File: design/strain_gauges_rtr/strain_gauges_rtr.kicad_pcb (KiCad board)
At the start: 2 copper layers, 88.9 x 44.5 mm, 41 parts, among them J1 Conn_01x03, J2 Conn_01x03, J3 Conn_01x08, J4 Conn_01x04, J5 Conn_01x04, J6 Conn_01x04, J7 Conn_01x04, P1 CONN_01X02, Q1 2N3096, U1 TL780-15, U2 LT1460-10, U3 INA826, U4 INA826, U5 INA826, U6 INA826

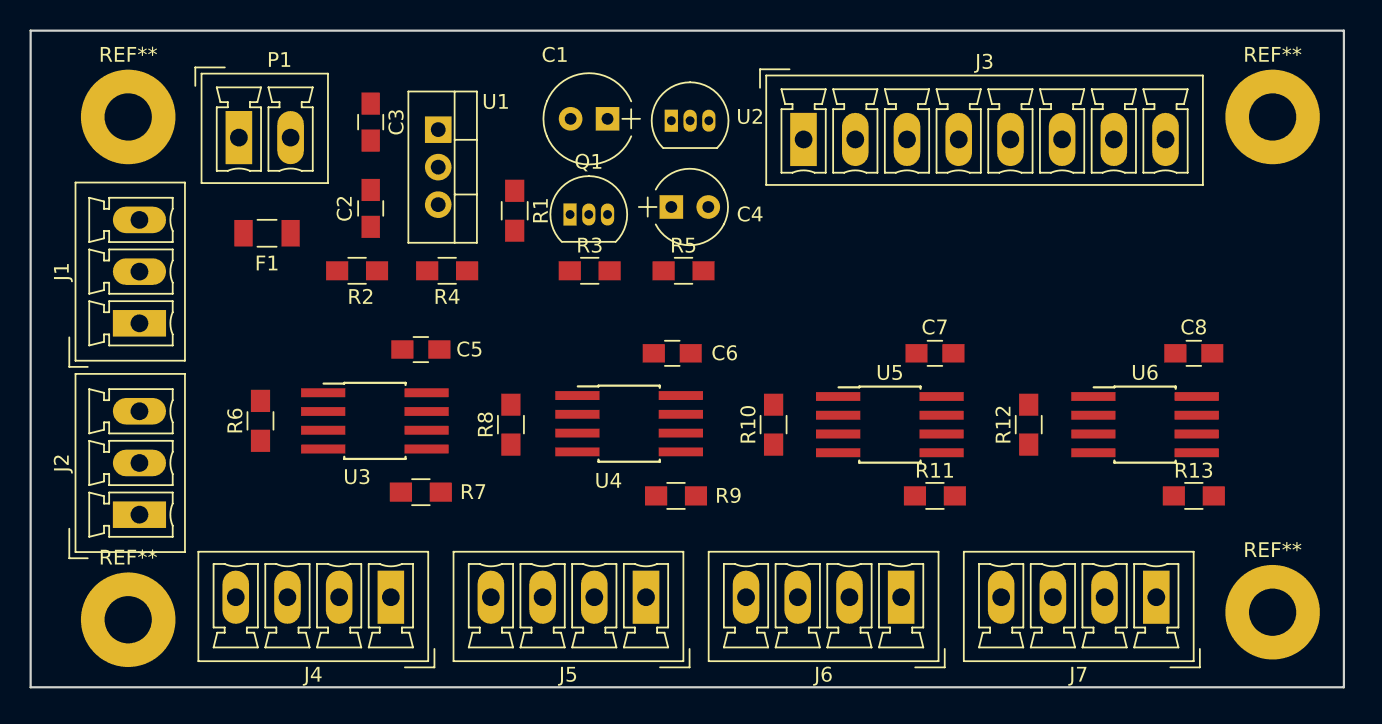
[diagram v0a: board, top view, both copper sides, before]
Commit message: Finish routing on INA826 board.
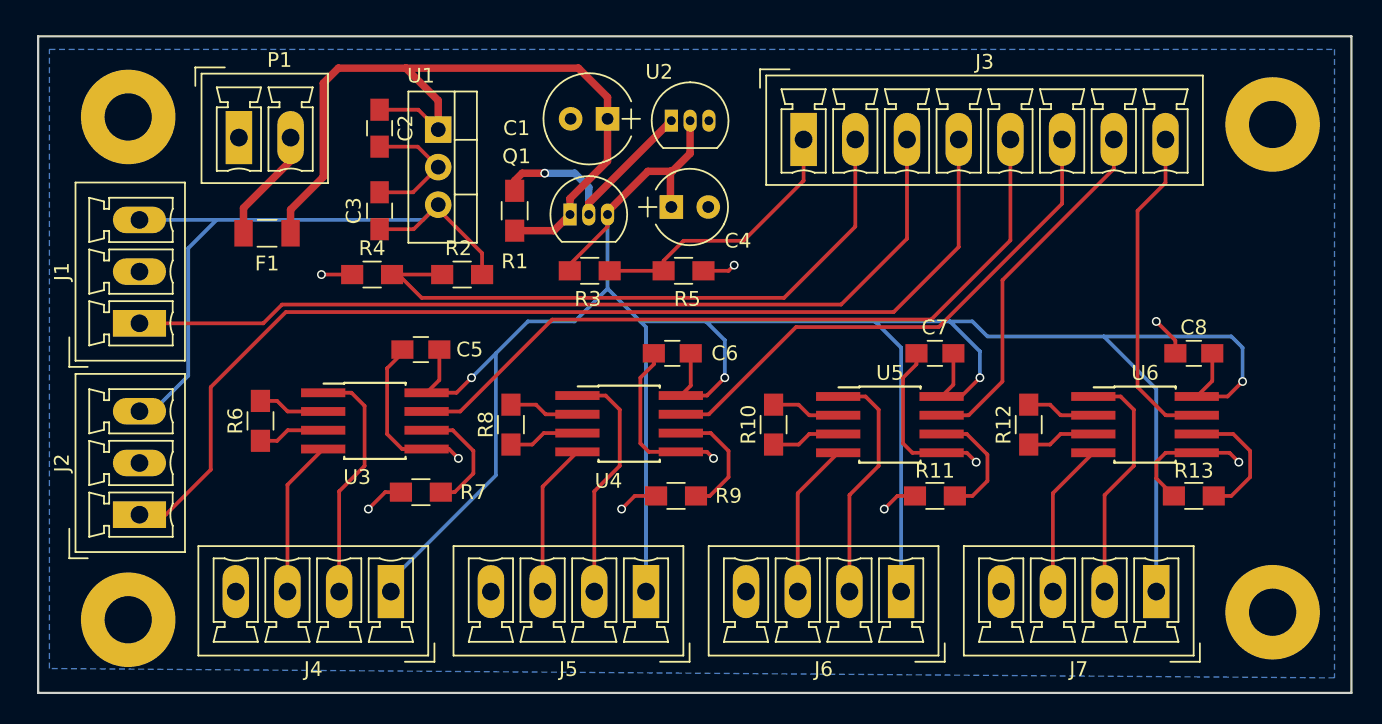
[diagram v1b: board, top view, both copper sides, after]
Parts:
- moved R2 7.12 mm to (118.4, 105.9), turned to 180 degrees
- moved C3 6.03 mm to (112.8, 101.6), turned to 90 degrees
- moved C2 5.46 mm to (112.8, 96.0), turned to 270 degrees
- moved R4 5.09 mm to (112.3, 105.9), turned to 180 degrees
- moved REF** 0.51 mm to (173.2, 95.8)
- moved J4 0.38 mm to (113.5, 127.4)
- moved J5 0.38 mm to (130.8, 127.4)
- moved J6 0.38 mm to (148.1, 127.4)
- moved J7 0.38 mm to (165.4, 127.4)
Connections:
- J3 pad 3: /PRESSURE_2 -> /PRESSURE_1
- J3 pad 4: /PRESSURE_1 -> /PRESSURE_2
- J3 pad 5: /STRAIN_OUT_4 -> /STRAIN_OUT_1
- J3 pad 6: /STRAIN_OUT_3 -> /STRAIN_OUT_2
- J3 pad 7: /STRAIN_OUT_2 -> /STRAIN_OUT_3
- J3 pad 8: /STRAIN_OUT_1 -> /STRAIN_OUT_4
- U4 pad 7: /STRAIN_OUT_3 -> /STRAIN_OUT_2
- U5 pad 7: /STRAIN_OUT_2 -> /STRAIN_OUT_3
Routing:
- net +10V: track 0.00 -> 191.5 mm, vias 0 -> 4
- net /PRESSURE_2: track 0.00 -> 73.5 mm
- net GND: track 0.00 -> 68.4 mm, vias 0 -> 10
- net /PRESSURE_1: track 0.00 -> 61.0 mm
- net +16V: track 0.00 -> 54.3 mm
- net /STRAIN_OUT_1: track 0.00 -> 51.1 mm
- net +15V: track 0.00 -> 46.9 mm
- net Net-(J3-Pad2): track 0.00 -> 43.3 mm
- net /STRAIN_OUT_2: track 0.00 -> 36.1 mm
- net /STRAIN_OUT_3: track 0.00 -> 24.6 mm
- net /STRAIN_OUT_4: track 0.00 -> 22.3 mm
- net Net-(J3-Pad1): track 0.00 -> 18.8 mm
- net Net-(Q1-Pad2): track 0.00 -> 16.8 mm, vias 0 -> 1
- net Net-(J4-Pad2): track 0.00 -> 16.5 mm
- net Net-(J5-Pad2): track 0.00 -> 16.3 mm
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- added copper zone on B.Cu, net GND
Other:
- rule pad_to_mask_clearance: 0.2 -> 0.1016
